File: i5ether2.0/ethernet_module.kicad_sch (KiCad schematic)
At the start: 14 parts, among them J2 Conn_02x05_Odd_Even, J3 1-406541-1, T2 HX5008

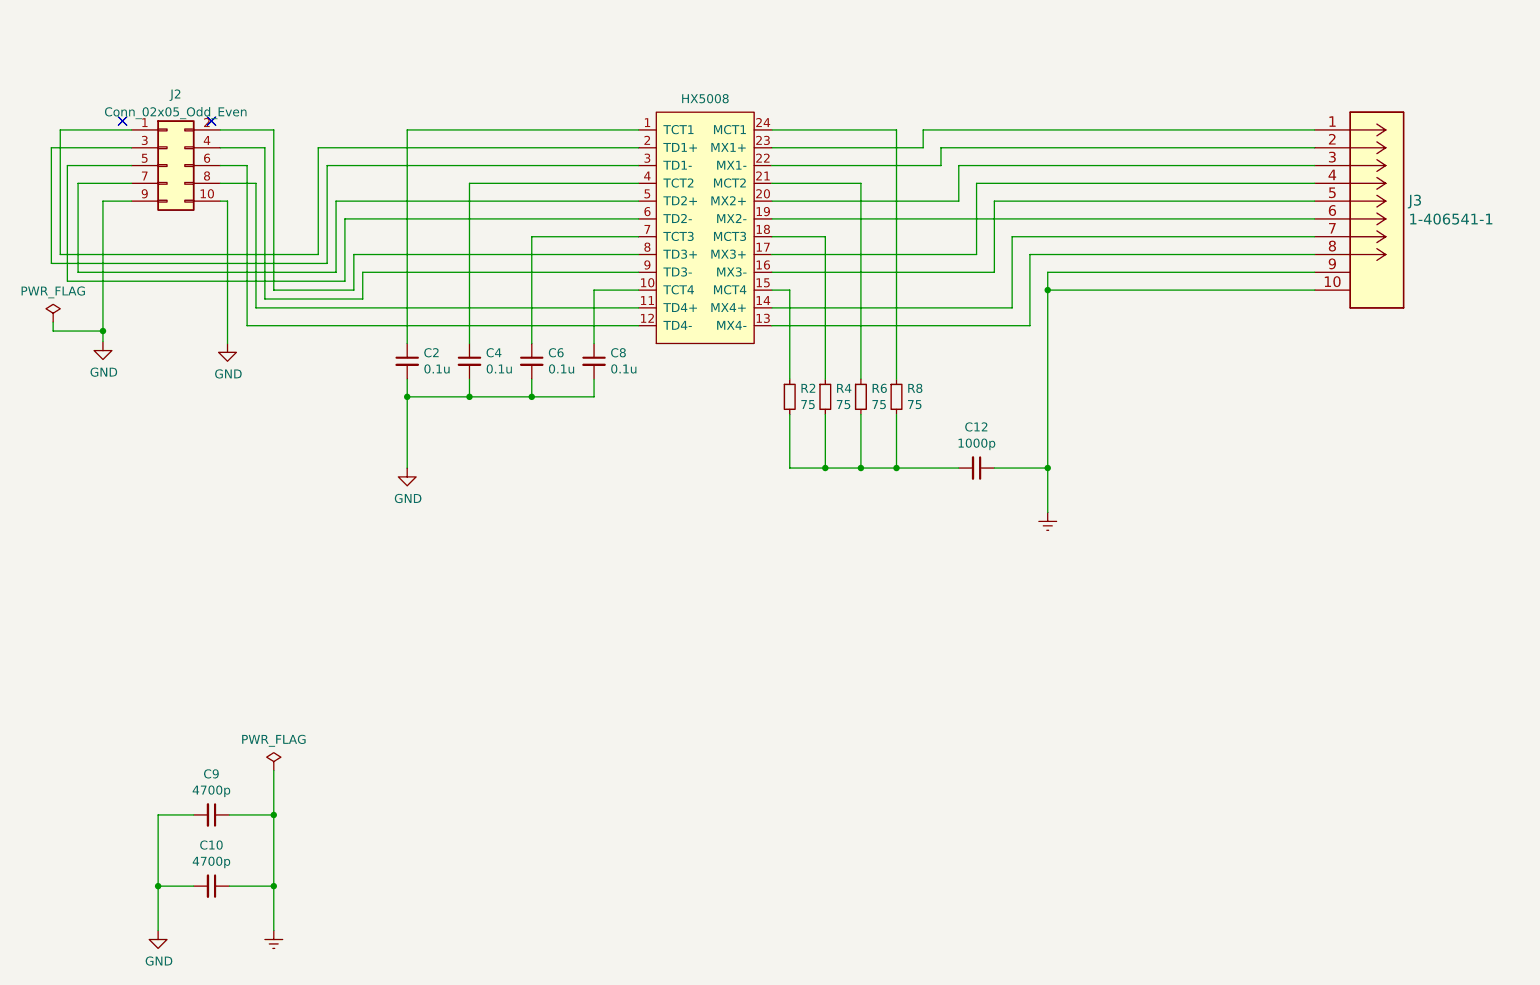
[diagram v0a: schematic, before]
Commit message: Essquematico con pantalla
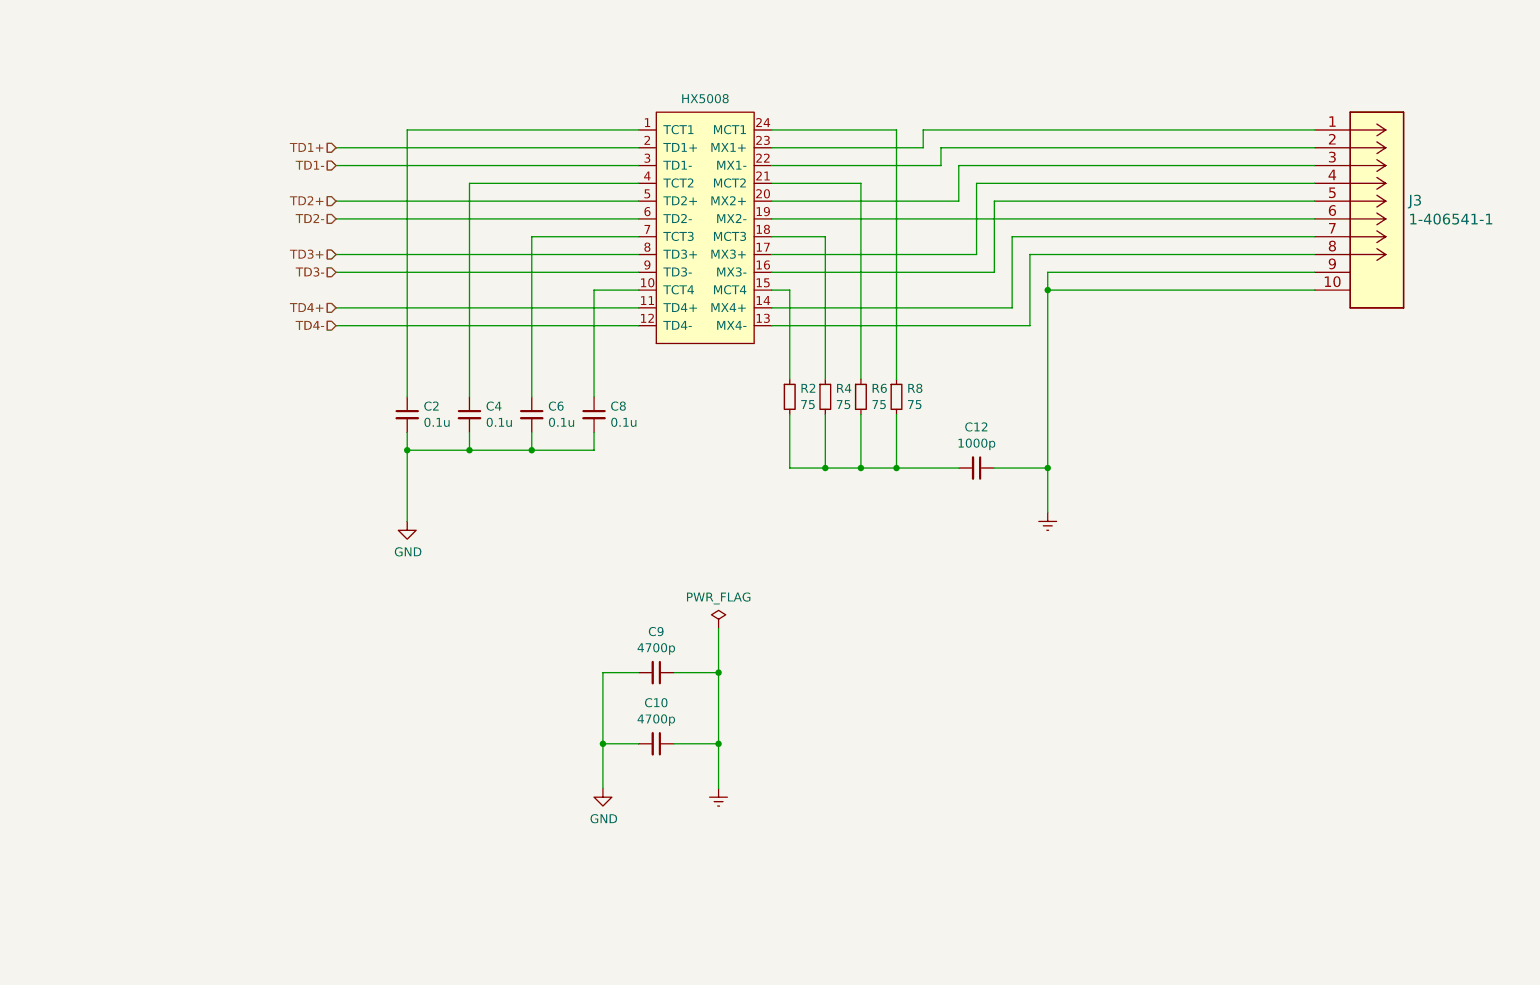
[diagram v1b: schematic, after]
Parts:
- removed J2: Conn_02x05_Odd_Even, Connector_PinHeader_2.54mm:PinHeader_2x05_P2.54mm_Vertical, symbol Connector_Generic:Conn_02x05_Odd_Even
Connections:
- net TD1+: now reaches T2.2 (TD1+)
- net TD3+: now reaches T2.8 (TD3+)
- net TD1-: now reaches T2.3 (TD1-)
- net TD3-: now reaches T2.9 (TD3-)
- net TD2-: now reaches T2.6 (TD2-)
- net TD4-: now reaches T2.12 (TD4-)
- net TD2+: now reaches T2.5 (TD2+)
- net TD4+: now reaches T2.11 (TD4+)
- no-connect marks 2 -> 0
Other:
- moved on the sheet: C10, C2, C4, C6, C8, C9

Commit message: Avances en placa
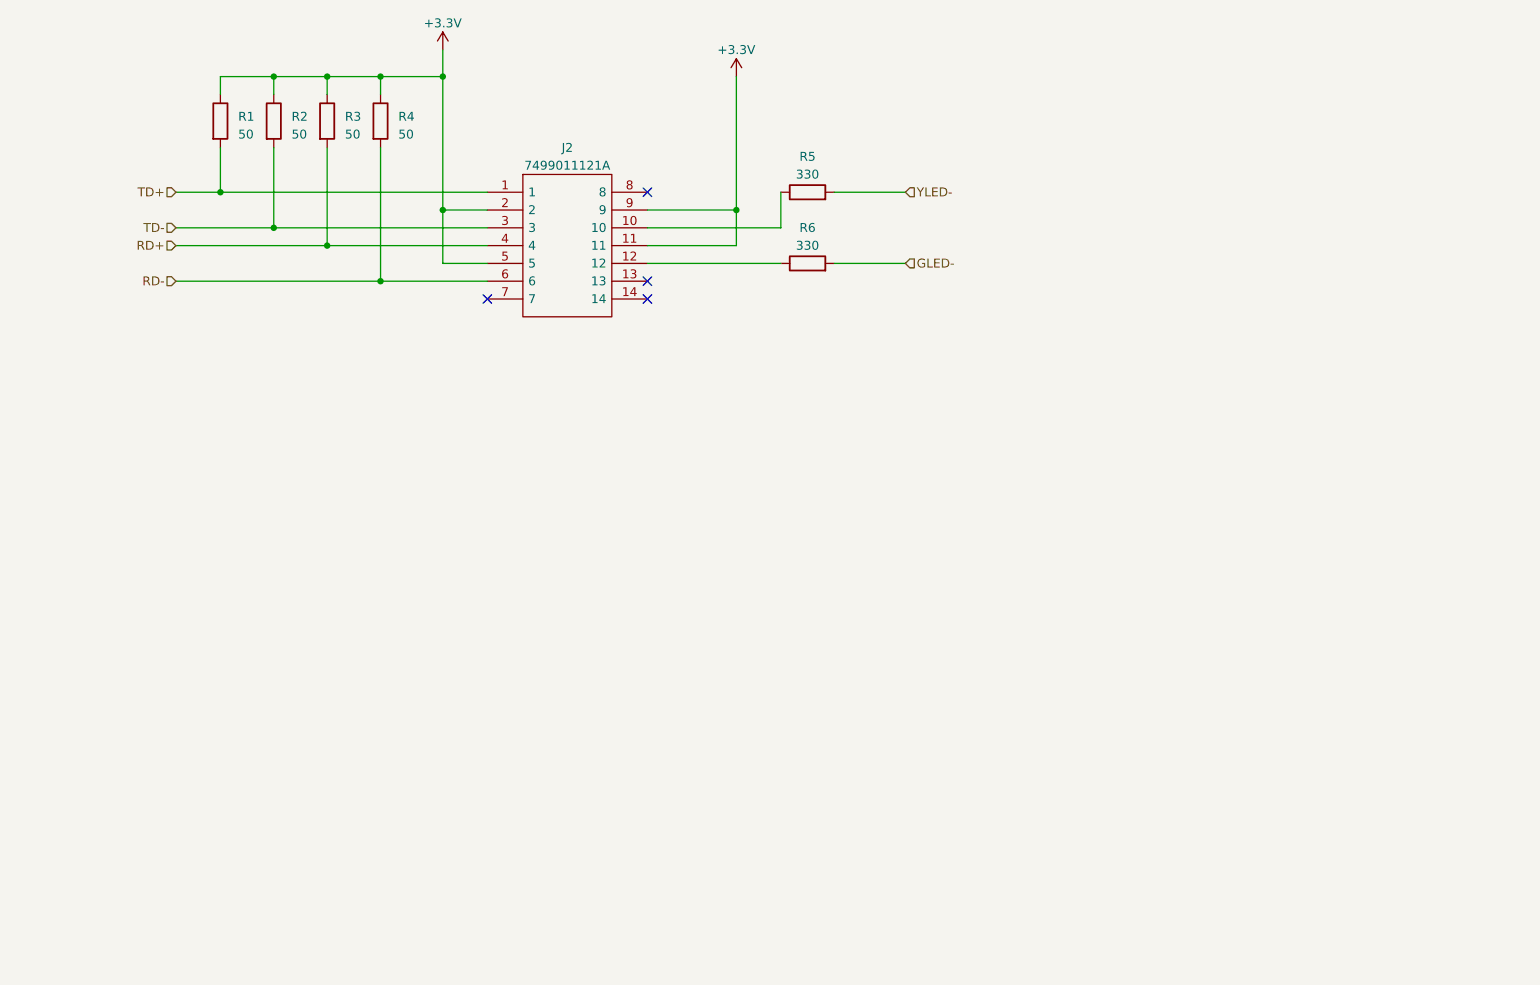
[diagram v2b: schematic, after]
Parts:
- removed C10, C9: 4700p, Resistor_SMD:R_1812_4532Metric, symbol Device:C_Small
- removed C12: 1000p, Capacitor_SMD:C_0402_1005Metric, symbol Device:C_Small
- removed C2, C4, C6, C8: 0.1u, Capacitor_SMD:C_0402_1005Metric, symbol Device:C_Small
- removed J3: 1-406541-1, MJ406541:1-406541-1, symbol MJ406541:1-406541-1
- removed R2, R4, R6, R8: 75, Resistor_SMD:R_0402_1005Metric, symbol Device:R_Small
- removed T2: HX5008, HX5008:HX5008NL, symbol HX5008:HX5008
- added J2: 7499011121A, KiCad:7499011121A, symbol 7499011121A:7499011121A
- added R1, R2, R3, R4: 50, symbol Device:R
- added R5, R6: 330, symbol Device:R
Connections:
- new net: J2.12, R6.1
- new net: J2.10, R5.1
- new net +3.3V: J2.11, J2.2, J2.5, J2.9, R1.1, R2.1, R3.1, R4.1
- new net GLED-: R6.2
- new net RD+: J2.4, R3.2
- new net RD-: J2.6, R4.2
- new net TD+: J2.1, R1.2
- new net TD-: J2.3, R2.2
- new net YLED-: R5.2
- no-connect marks 0 -> 4
